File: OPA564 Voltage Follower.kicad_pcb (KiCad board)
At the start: 2 copper layers, 70 x 45 mm, 20 parts, among them IC1 OPA564AIDWD, IC2 OPA564AIDWD, J1 Conn_Coaxial, J2 Conn_Coaxial

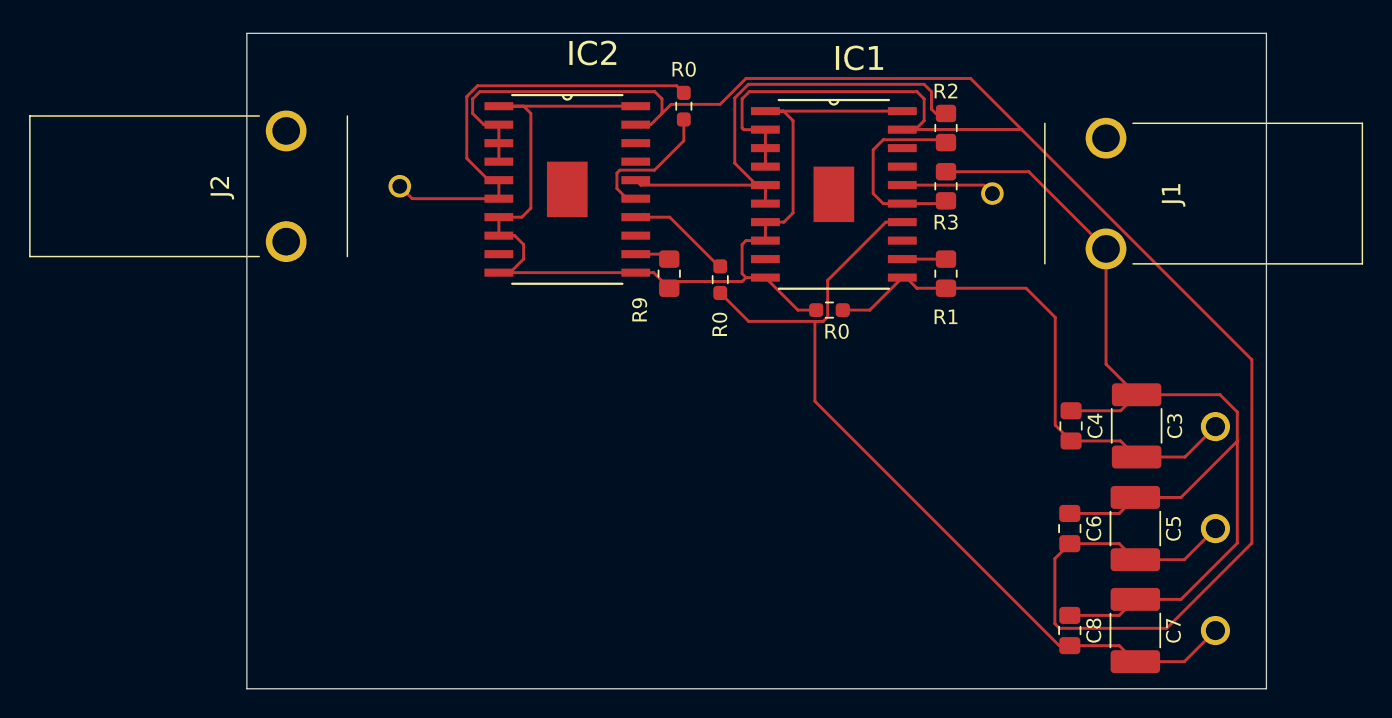
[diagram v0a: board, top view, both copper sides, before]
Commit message: version 1 i guess
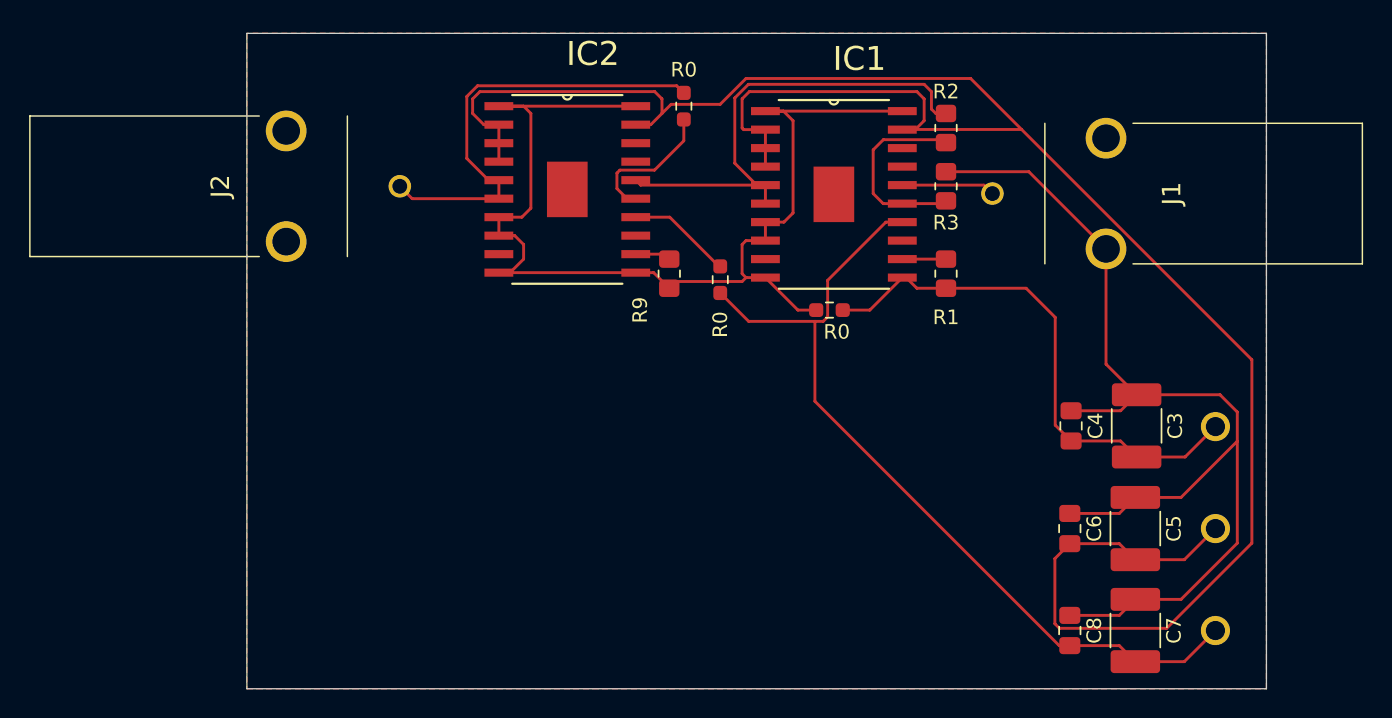
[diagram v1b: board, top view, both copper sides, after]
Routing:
- added copper zone on F.Cu, net GND
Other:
- board text removed: "Function Amplifier w/ Voltage Follower Andy Yang"
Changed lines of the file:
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@@
 		(layer "Edge.Cuts")
-	)
-	(gr_text "Function Amplifier w/ Voltage Follower\nAndy Yang\n"
-		(at 134 88.5 0)
-		(layer "Edge.Cuts")
-		(effects
-			(font
-				(size 1 1)
-				(thickness 0.15)
-			)
-			(justify left bottom)
-		)
 	)
 	(segment
@@
 		(net "Net-(IC2-ISET)")
 	)
+	(zone
+		(net "GND")
+		(layer "F.Cu")
+		(hatch edge 0.5)
+		(connect_pads
+			(clearance 0.5)
+		)
+		(min_thickness 0.25)
+		(fill yes
+			(thermal_gap 0.5)
+			(thermal_bridge_width 0.5)
+			(island_removal_mode 0)
+		)
+		(polygon
+			(pts
+				(xy 202.5 90) (xy 202.5 45) (xy 132.5 45) (xy 132.5 90)
+			)
+		)
+	)
 	(embedded_fonts no)
